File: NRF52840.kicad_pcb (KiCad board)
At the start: 2 copper layers, 31.2 x 11.3 mm, 26 parts, among them J1 Conn_01x04, J2 USB_A, U1 nRF52840, Y1 32M

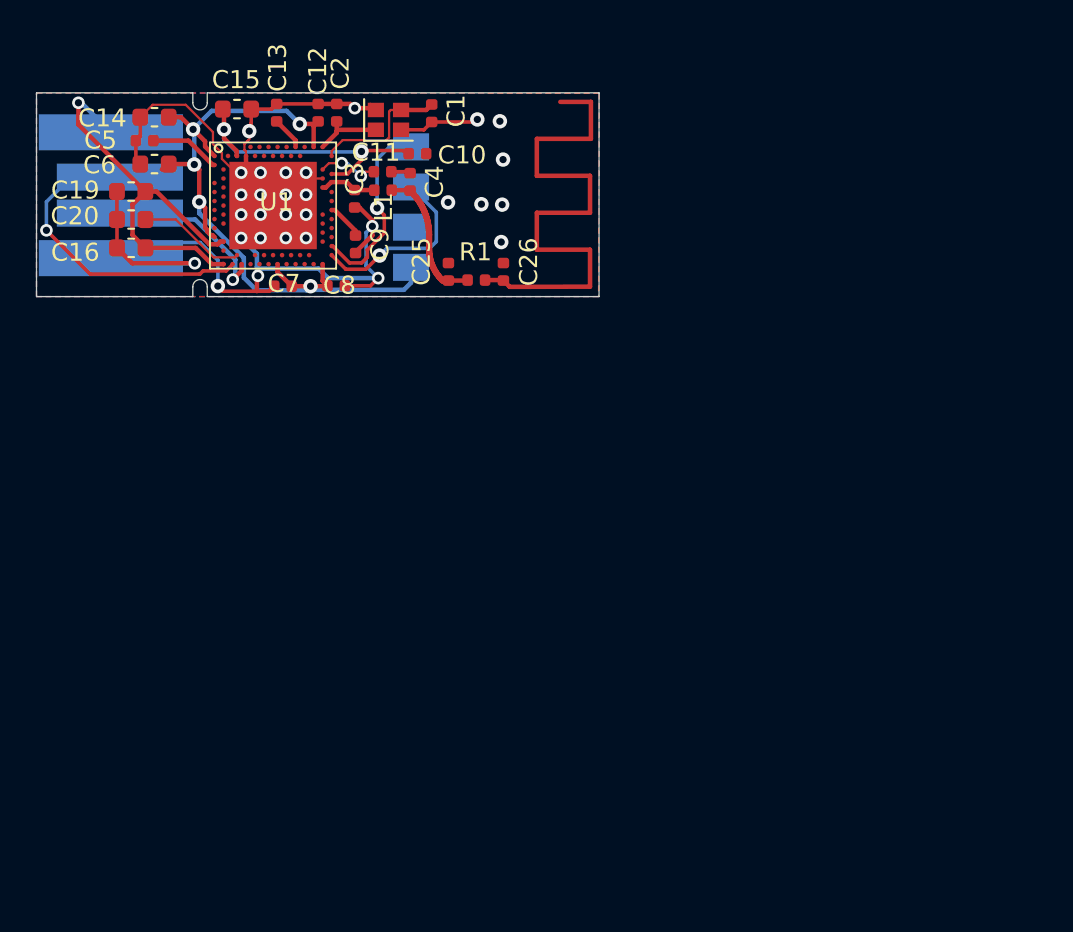
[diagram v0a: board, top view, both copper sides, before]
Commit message: ...
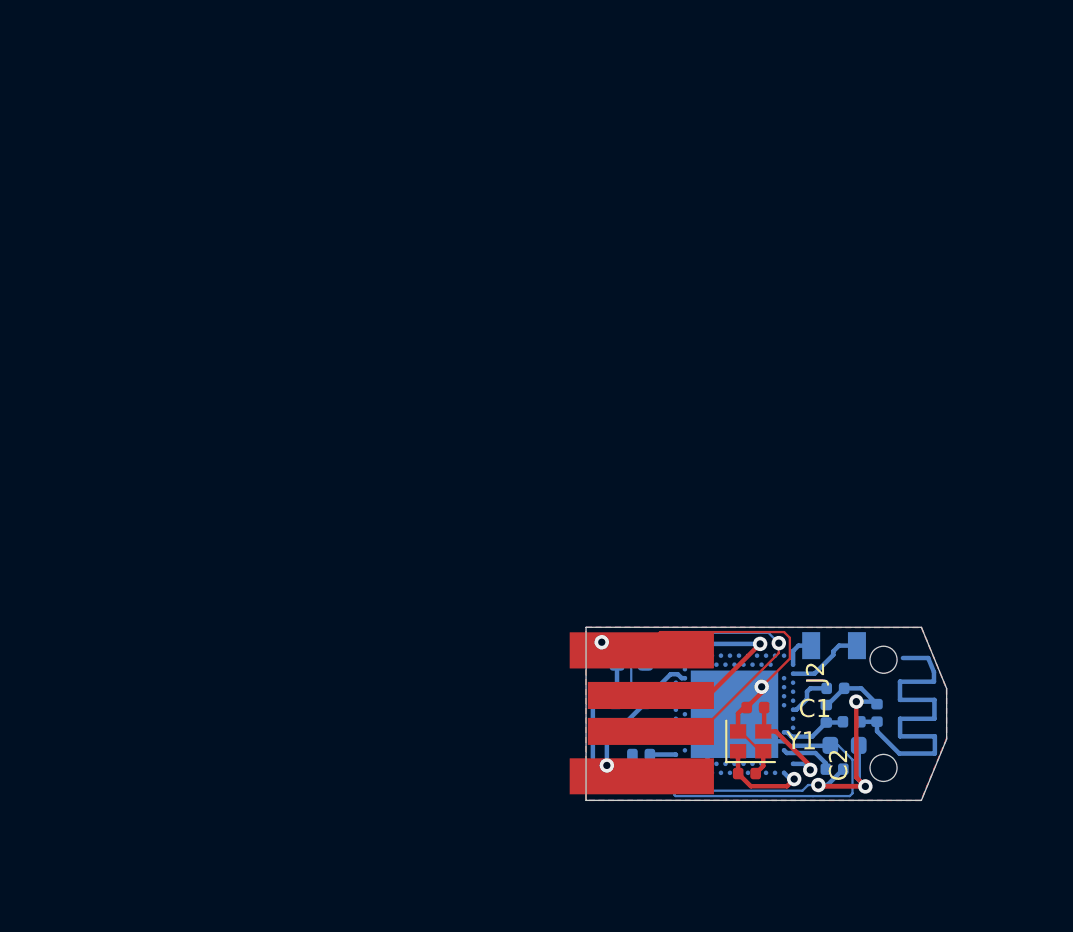
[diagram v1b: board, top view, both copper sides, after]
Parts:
- removed C10, C13, C25: NC, Capacitor_SMD:C_0402_1005Metric
- removed C12, C8: 100nF, Capacitor_SMD:C_0402_1005Metric
- removed C14: 1.0uF, Capacitor_SMD:C_0603_1608Metric
- removed C19, C6: 4.7uF, Capacitor_SMD:C_0603_1608Metric
- removed C26: 1.5pF, Capacitor_SMD:C_0402_1005Metric
- removed C7: 100nf, Capacitor_SMD:C_0402_1005Metric
- removed R1: 0R, Capacitor_SMD:C_0402_1005Metric
- C11, C15, C16, C20, C3, C4, C5, C9, L1, U1: moved to B.Cu
- J1: value Conn_01x04 -> Conn_01x02; footprint zhangxiaofei:SWD -> zhangxiaofei:SWD_2_PIN
- J2: moved to F.Cu
- moved C15 48.8 mm to (134.8, 156.9)
- moved C5 43.8 mm to (123.6, 157.4)
- moved C2 43.1 mm to (129.4, 158.5), turned to 180 degrees
- moved C11 41.5 mm to (134.3, 158.2)
- moved J2 40.5 mm to (124.4, 154.7), turned to 90 degrees
- moved Y1 39.9 mm to (129.6, 156.7)
- moved L1 39.3 mm to (135.2, 155.6)
- moved C4 39.2 mm to (136.6, 155.1)
- moved C3 38.7 mm to (133.8, 155.1), turned to 270 degrees
- moved U1 38.1 mm to (128.7, 155.2)
- moved C1 37.5 mm to (129.9, 154.8), turned to 0 degrees
- moved C16 37.4 mm to (122.9, 154.4)
- moved C20 37.0 mm to (123.0, 152.3)
- moved C9 36.3 mm to (134.3, 153.7), turned to 0 degrees
- moved J1 34.1 mm to (134.3, 151.4), turned to 180 degrees
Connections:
- U1 pad A10: Net-(U1-PadA10) -> (no net)
- U1 pad A12: Net-(U1-PadA12) -> (no net)
- U1 pad A14: Net-(U1-PadA14) -> (no net)
- U1 pad A16: Net-(U1-PadA16) -> (no net)
- U1 pad A18: Net-(C13-Pad2) -> (no net)
- U1 pad A20: Net-(U1-PadA20) -> (no net)
- U1 pad A22: +3V3 -> (no net)
- U1 pad A8: Net-(U1-PadA8) -> (no net)
- U1 pad AB2: Net-(U1-PadAB2) -> (no net)
- U1 pad AC11: Net-(U1-PadAC11) -> (no net)
- U1 pad AC13: Net-(U1-PadAC13) -> (no net)
- U1 pad AC15: Net-(U1-PadAC15) -> (no net)
- U1 pad AC17: Net-(U1-PadAC17) -> (no net)
- U1 pad AC19: Net-(U1-PadAC19) -> (no net)
- U1 pad AC21: Net-(U1-PadAC21) -> (no net)
- U1 pad AC9: Net-(U1-PadAC9) -> (no net)
- U1 pad AD10: Net-(U1-PadAD10) -> (no net)
- U1 pad AD12: Net-(U1-PadAD12) -> (no net)
- U1 pad AD14: +3V3 -> (no net)
- U1 pad AD16: Net-(U1-PadAD16) -> (no net)
- U1 pad AD18: Net-(U1-PadAD18) -> (no net)
- U1 pad AD20: Net-(U1-PadAD20) -> (no net)
- U1 pad AD22: Net-(U1-PadAD22) -> (no net)
- U1 pad AD23: +3V3 -> (no net)
- U1 pad AD8: Net-(U1-PadAD8) -> (no net)
- U1 pad B1: +3V3 -> (no net)
- U1 pad B11: Net-(U1-PadB11) -> (no net)
- U1 pad B13: Net-(U1-PadB13) -> (no net)
- U1 pad B15: Net-(U1-PadB15) -> (no net)
- U1 pad B17: Net-(U1-PadB17) -> (no net)
- U1 pad B19: Net-(U1-PadB19) -> (no net)
- U1 pad B3: Net-(U1-PadB3) -> (no net)
- U1 pad B9: Net-(U1-PadB9) -> (no net)
- U1 pad D2: Net-(U1-PadD2) -> (no net)
- U1 pad F2: Net-(U1-PadF2) -> (no net)
- U1 pad G1: Net-(U1-PadG1) -> (no net)
- U1 pad H2: Net-(U1-PadH2) -> (no net)
- U1 pad J1: Net-(U1-PadJ1) -> (no net)
- U1 pad J24: Net-(U1-PadJ24) -> (no net)
- U1 pad K2: Net-(U1-PadK2) -> (no net)
- U1 pad L1: Net-(U1-PadL1) -> (no net)
- U1 pad L24: Net-(U1-PadL24) -> (no net)
- U1 pad M2: Net-(U1-PadM2) -> (no net)
- U1 pad N1: Net-(U1-PadN1) -> (no net)
- U1 pad P2: Net-(U1-PadP2) -> (no net)
- U1 pad P23: Net-(U1-PadP23) -> (no net)
- U1 pad R1: Net-(U1-PadR1) -> (no net)
- U1 pad R24: Net-(U1-PadR24) -> (no net)
- U1 pad T2: Net-(U1-PadT2) -> (no net)
- U1 pad T23: Net-(U1-PadT23) -> (no net)
- U1 pad U1: Net-(U1-PadU1) -> (no net)
- U1 pad U24: Net-(U1-PadU24) -> (no net)
- U1 pad V23: Net-(U1-PadV23) -> (no net)
- U1 pad W1: +3V3 -> (no net)
- U1 pad W24: Net-(U1-PadW24) -> (no net)
- U1 pad Y23: Net-(U1-PadY23) -> (no net)
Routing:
- net +3V3: track 42.5 -> 0.00 mm, vias 5 -> 0
- net Net-(AE1-Pad1) (its old number): track 29.8 -> 0.00 mm
- net +5V: track 35.3 -> 13.8 mm
- net GND: track 79.6 -> 67.5 mm, vias 30 -> 5
- net Net-(AE1-Pad1): track 7.90 -> 19.6 mm
- net SWDIO: track 10.4 -> 1.88 mm, vias 1 -> 0
- net SWDCLK: track 10.7 -> 4.30 mm, vias 1 -> 0
- net D+: track 6.31 -> 10.8 mm
- net Net-(C20-Pad1): track 6.00 -> 3.00 mm
- net D-: track 17.8 -> 15.0 mm
- net Net-(C5-Pad1): track 3.95 -> 1.45 mm
- net Net-(C13-Pad2): track 1.85 -> 0.00 mm
- net Net-(C1-Pad2): track 7.76 -> 6.09 mm, vias 0 -> 1
- net Net-(C2-Pad2): track 3.94 -> 5.51 mm, vias 0 -> 1
- net Net-(C15-Pad1): track 16.5 -> 17.8 mm, vias 2 -> 0
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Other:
- board size 31.2 x 11.3 mm -> 20 x 9.6 mm
- board text added: "c"
- board text added: "i"
- board text removed: "3V3"
- board text removed: "5"
- board text removed: "D+"
- board text removed: "D-"
- board text removed: "GND"
- board text removed: "SWDCLK"
- board text removed: "SWDIO"

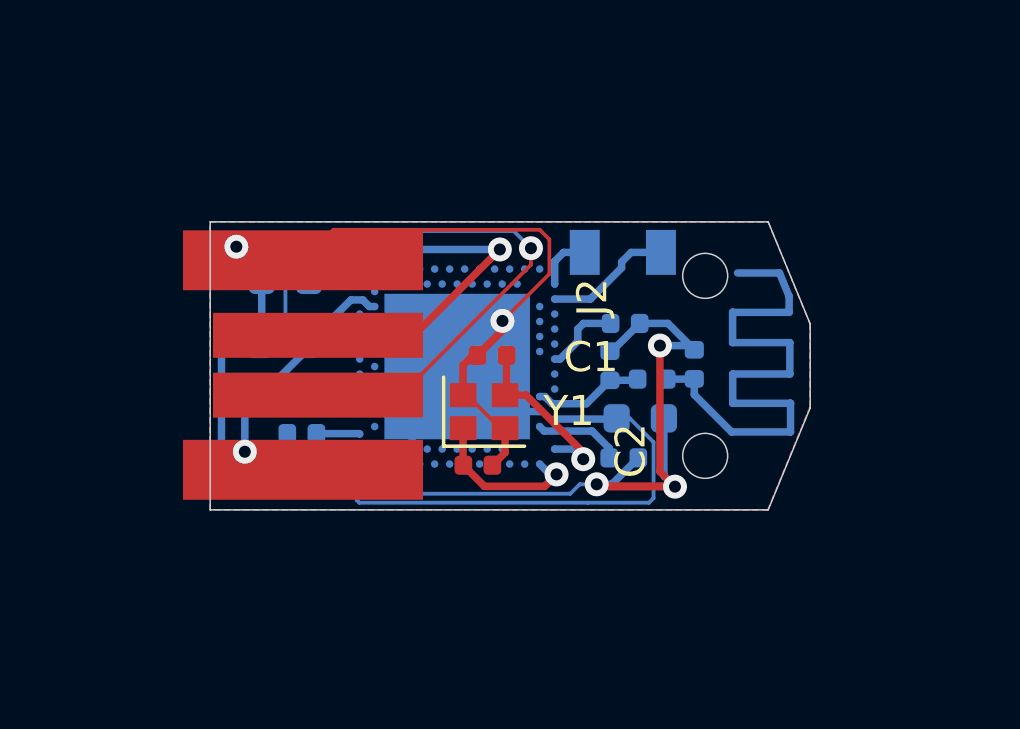
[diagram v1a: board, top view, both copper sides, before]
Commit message: ...
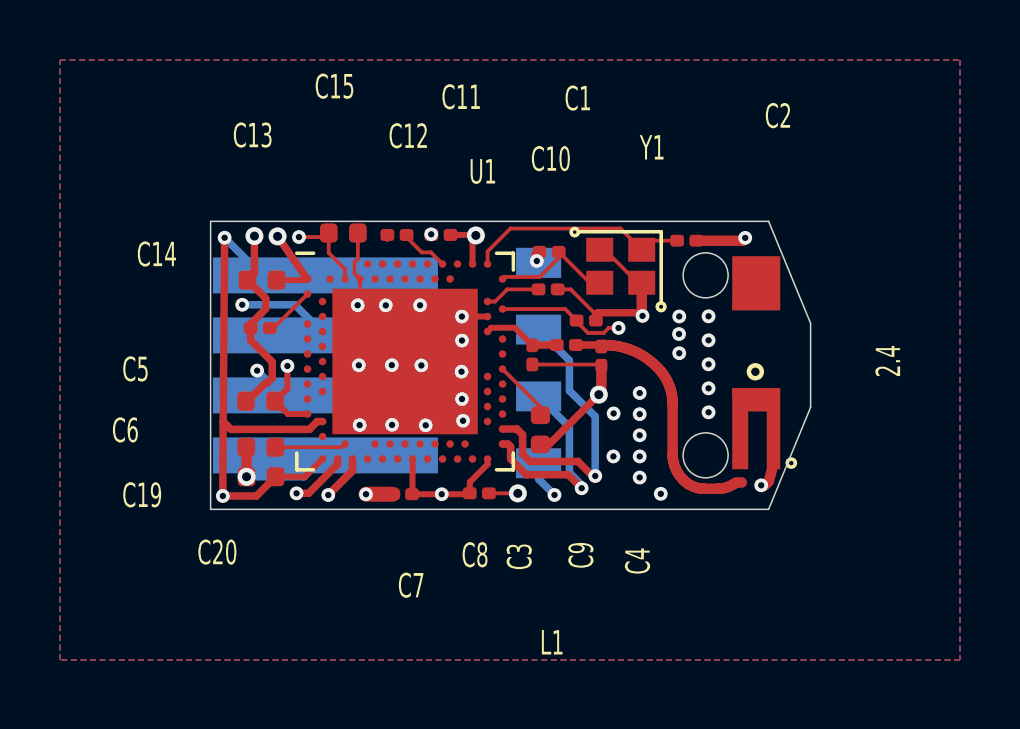
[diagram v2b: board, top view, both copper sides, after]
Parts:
- removed C16: 4.7uF, Capacitor_SMD:C_0603_1608Metric
- added 2.4: 2.4g_taocitianxian, zhangxiaofei:2.4g_taocitianxian, F.Cu at (138.8, 154.7)
- added C10: NC, Capacitor_SMD:C_0201_0603Metric, F.Cu at (133.0, 153.6)
- added C12: 100nF, Capacitor_SMD:C_0201_0603Metric, F.Cu at (128.2, 150.8)
- added C13: NC, Capacitor_SMD:C_0201_0603Metric, F.Cu at (126.7, 150.8)
- added C14: 1.0uf, Capacitor_SMD:C_0402_1005Metric, F.Cu at (122.2, 152.3)
- added C19: 4.7uF, Capacitor_SMD:C_0402_1005Metric, F.Cu at (122.2, 158.8)
- added C6: 4.7uF, Capacitor_SMD:C_0402_1005Metric, F.Cu at (122.2, 156.3)
- added C7: 100nF, Capacitor_SMD:C_0201_0603Metric, F.Cu at (126.9, 159.4)
- added C8: 100nF, Capacitor_SMD:C_0201_0603Metric, F.Cu at (129.5, 159.4)
- C1, C2: footprint Capacitor_SMD:C_0402_1005Metric -> Capacitor_SMD:C_0201_0603Metric
- C11, C5: footprint Capacitor_SMD:C_0402_1005Metric -> Capacitor_SMD:C_0201_0603Metric; moved to F.Cu
- C15, C20: footprint Capacitor_SMD:C_0603_1608Metric -> Capacitor_SMD:C_0402_1005Metric; moved to F.Cu
- C3: value 1.0pF -> 0.8pF; footprint Capacitor_SMD:C_0402_1005Metric -> Capacitor_SMD:C_0201_0603Metric; moved to F.Cu
- C4: value 1.0pF -> 0.5pF; footprint Capacitor_SMD:C_0402_1005Metric -> Capacitor_SMD:C_0201_0603Metric; moved to F.Cu
- C9, U1: moved to F.Cu
- J1: value Conn_01x02 -> Conn_01x04; footprint zhangxiaofei:SWD_2_PIN -> zhangxiaofei:SWD
- J2: footprint zhangxiaofei:USB_PCB -> zhangxiaofei:mini_usb; moved to B.Cu
- L1: value 3.9nH -> 4.7nH; footprint Inductor_SMD:L_0402_1005Metric -> Inductor_SMD:L_0201_0603Metric; moved to F.Cu
- moved C15 11.7 mm to (124.9, 150.7)
- moved C2 10.2 mm to (136.4, 151.0)
- moved Y1 6.65 mm to (134.2, 151.8), turned to 180 degrees
- moved C11 6.16 mm to (131.8, 152.6)
- moved C20 5.64 mm to (122.2, 157.9)
- moved C9 4.53 mm to (131.5, 157.3), turned to 270 degrees
- moved J1 4.33 mm to (131.4, 154.6), turned to 270 degrees
- moved C1 3.94 mm to (131.8, 151.3)
- moved C5 3.78 mm to (122.2, 153.9)
- moved C4 3.11 mm to (133.5, 154.8), turned to 270 degrees
- moved L1 3.08 mm to (132.4, 154.4)
- moved C3 2.61 mm to (131.2, 154.8), turned to 90 degrees
- moved U1 1.75 mm to (127.0, 155.0)
- moved J2 0.79 mm to (124.3, 155.5), turned to 270 degrees
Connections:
- J1 pad 1: SWDCLK -> GND
- J1 pad 2: SWDIO -> SWDCLK
- U1 pad A18: (no net) -> Net-(C13-Pad1)
- U1 pad A22: (no net) -> +3V3
- U1 pad AD14: (no net) -> +3V3
- U1 pad AD23: (no net) -> +3V3
- U1 pad B1: (no net) -> +3V3
- U1 pad W1: (no net) -> +3V3
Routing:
- net GND: track 67.5 -> 36.4 mm, vias 5 -> 40
- net +3V3: track 0.00 -> 13.3 mm, vias 0 -> 5
- net Net-(AE1-Pad1): track 19.6 -> 8.92 mm
- net +5V: track 13.8 -> 19.9 mm, vias 1 -> 2
- net SWDCLK: track 4.30 -> 9.78 mm, vias 0 -> 1
- net SWDIO: track 1.88 -> 7.14 mm, vias 0 -> 1
- net D-: track 15.0 -> 12.4 mm, vias 1 -> 2
- net Net-(C2-Pad2): track 5.51 -> 7.47 mm, vias 1 -> 0
- net Net-(C1-Pad2): track 6.09 -> 4.16 mm, vias 1 -> 0
- net Net-(C13-Pad1): track 0.00 -> 1.64 mm
- net Net-(C10-Pad2): track 17.8 -> 19.4 mm, vias 0 -> 2
- net Net-(C3-Pad2): track 3.70 -> 2.61 mm
- net Net-(C11-Pad2): track 2.94 -> 1.87 mm
- net Net-(C20-Pad1): track 3.00 -> 2.37 mm
- net Net-(C9-Pad1): track 2.59 -> 2.07 mm
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- added copper zone on VCC2.Cu, net +3V3
- added copper zone on GND1.Cu, net GND
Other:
- outline, holes or cut-outs redrawn
- copper layers 2 -> 4
- rule via_min_drill: 0.3 -> 0.2
- rule via_min_size: 0.4 -> 0.2
- board text added: "3.3"
- board text added: "CLK"
- board text added: "GND"
- board text added: "IO"
- board text removed: "c"
- board text removed: "i"
